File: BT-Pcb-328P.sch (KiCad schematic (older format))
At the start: 18 parts, among them J1 USB_B_Micro, P1 MYSX_2.6, Q1 FDN338P, SW1 1437566-3, U1 AMS1117-3.3, U2 AS312, U3 ATmega328P-AU, U4 RFM69HW

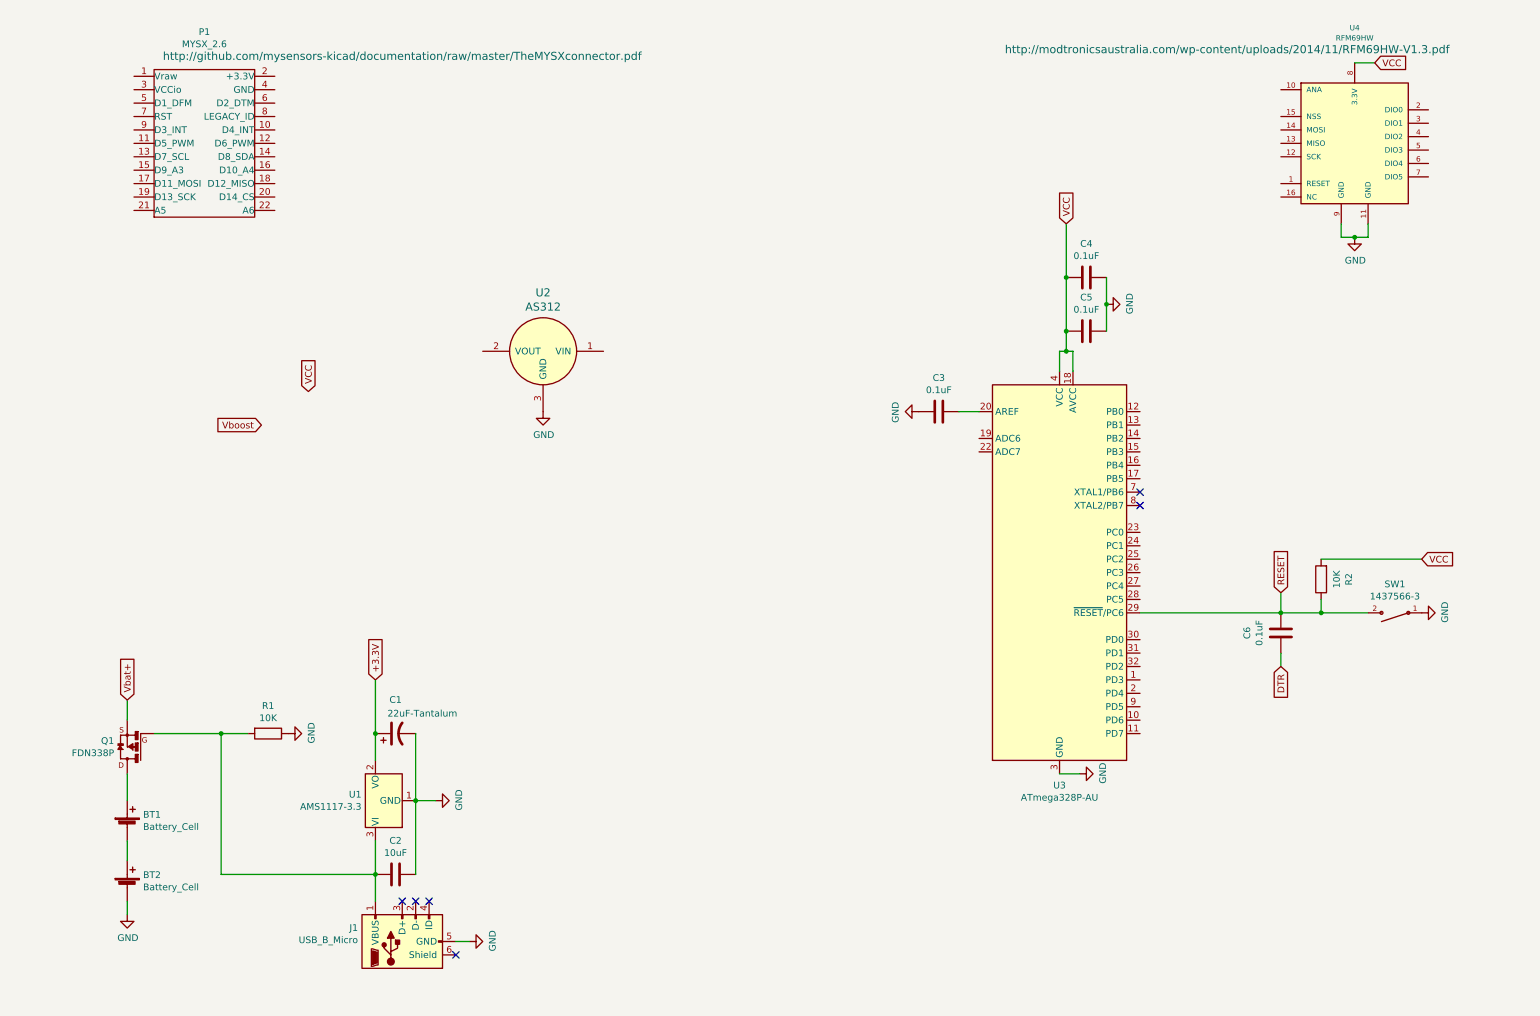
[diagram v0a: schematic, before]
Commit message: Development 2
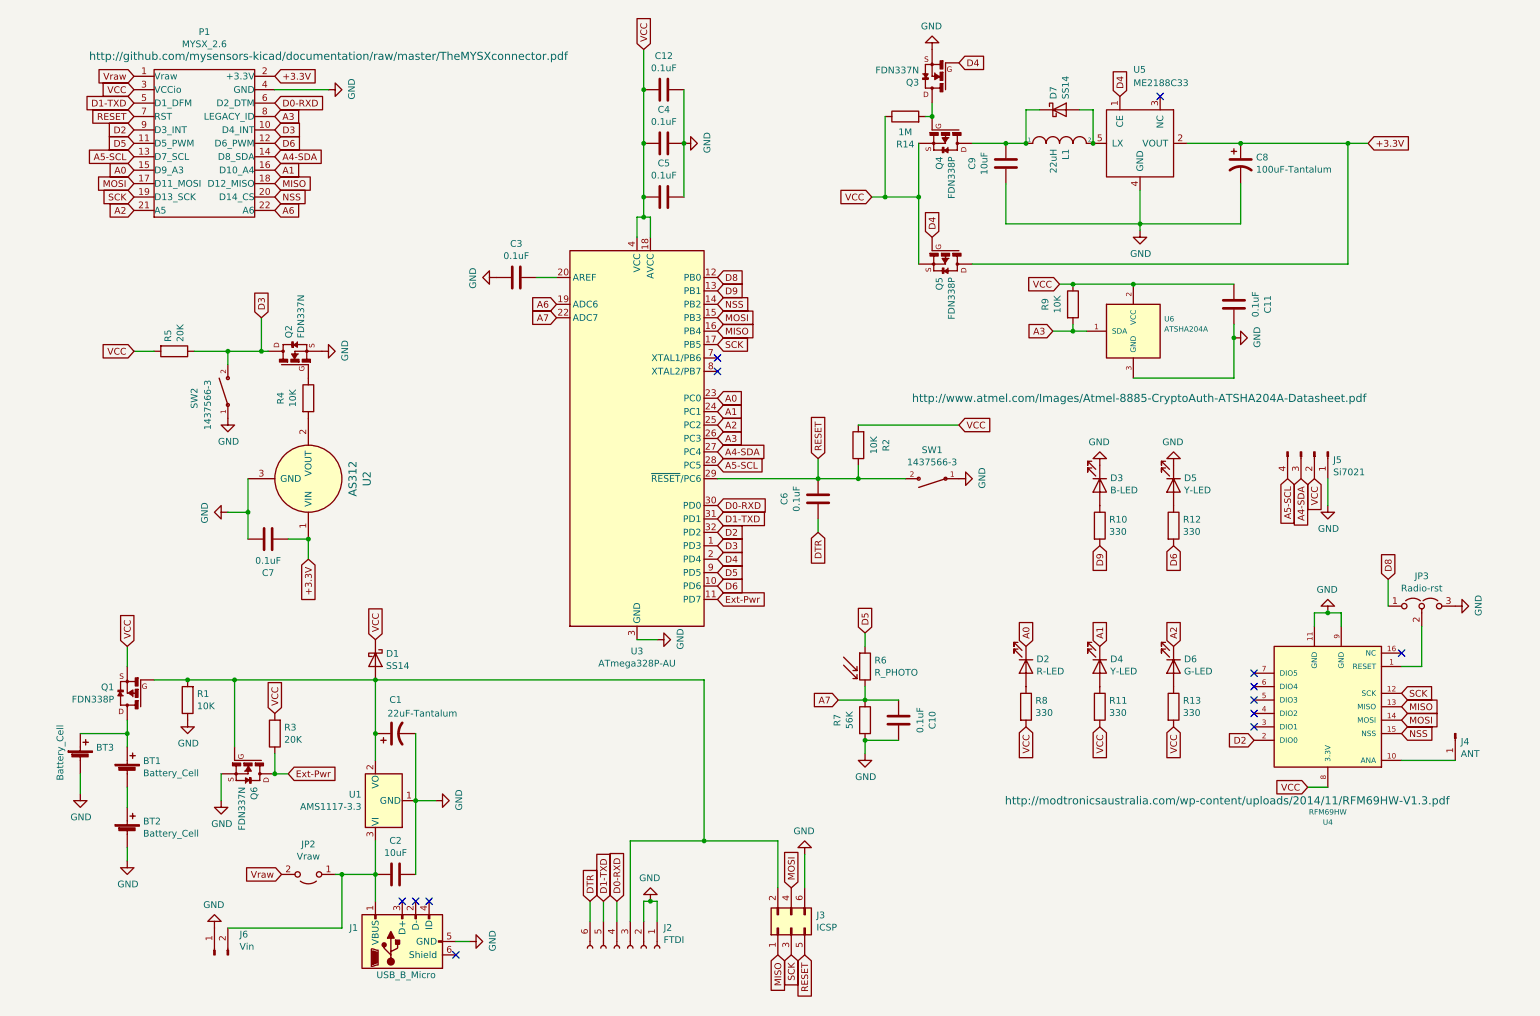
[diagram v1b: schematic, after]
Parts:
- added BT3: Battery_Cell, Battery:BatteryHolder_Keystone_1058_1x2032, symbol Device:Battery_Cell
- added C10, C11, C12, C7: 0.1uF, Capacitor_SMD:C_0805_2012Metric, symbol Device:C
- added C8: 100uF-Tantalum, capacitors:TAJD107K016RNJV, symbol Device:CP1
- added C9: 10uF, Capacitor_SMD:C_0805_2012Metric, symbol Device:C
- added D1, D7: SS14, diodes:SS14, symbol Device:D_Schottky
- added D2: R-LED, LED_SMD:LED_0805_2012Metric, symbol Device:LED
- added D3: B-LED, LED_SMD:LED_0805_2012Metric, symbol Device:LED
- added D4, D5: Y-LED, LED_SMD:LED_0805_2012Metric, symbol Device:LED
- added D6: G-LED, LED_SMD:LED_0805_2012Metric, symbol Device:LED
- added J2: FTDI, Connector_PinSocket_2.54mm:PinSocket_1x06_P2.54mm_Vertical, symbol Connector:Conn_01x06_Female
- added J3: ICSP, Connector_PinHeader_2.54mm:PinHeader_2x03_P2.54mm_Vertical, symbol Connector_Generic:Conn_02x03_Odd_Even
- added J4: ANT, Connector_PinHeader_2.54mm:PinHeader_1x01_P2.54mm_Vertical, symbol Connector:Conn_01x01_Male
- added J5: Si7021, Connector_PinHeader_2.54mm:PinHeader_1x04_P2.54mm_Vertical, symbol Connector:Conn_01x04_Male
- added J6: Vin, Connector_PinHeader_2.54mm:PinHeader_1x02_P2.54mm_Vertical, symbol Connector:Conn_01x02_Male
- added JP2: Vraw, Jumper:SolderJumper-2_P1.3mm_Open_RoundedPad1.0x1.5mm, symbol Jumper:Jumper_2_Open
- added JP3: Radio-rst, Jumper:SolderJumper-3_P1.3mm_Open_RoundedPad1.0x1.5mm_NumberLabels, symbol Jumper:Jumper_3_Open
- added L1: 22uH, Inductor_SMD:L_6.3x6.3_H3, symbol pspice:INDUCTOR
- added Q2, Q3, Q6: FDN337N, FDN337N:SSOT-3, symbol FDN337N:FDN337N
- added Q4, Q5: FDN338P, FDN338P:SSOT-3, symbol FDN338P:FDN338P
- added R10, R11, R12, R13, R8: 330, Resistor_SMD:R_0805_2012Metric, symbol Device:R
- added R14: 1M, Resistor_SMD:R_0805_2012Metric, symbol Device:R
- added R3, R5: 20K, Resistor_SMD:R_0805_2012Metric, symbol Device:R
- added R4, R9: 10K, Resistor_SMD:R_0805_2012Metric, symbol Device:R
- added R6: R_PHOTO, OptoDevice:R_LDR_5.0x4.1mm_P3mm_Vertical, symbol Device:R_PHOTO
- added R7: 56K, Resistor_SMD:R_0805_2012Metric, symbol Device:R
- added SW2: 1437566-3, 1437566-3:SW_1437566-3, symbol 1437566-3:1437566-3
- added U5: ME2188C33, Package_TO_SOT_SMD:SOT-23-5, symbol boost-converters:ME2188C33
- added U6: ATSHA204A, Package_TO_SOT_SMD:SOT-23_Handsoldering, symbol mysensors_security:ATSHA204A
- BT1, BT2: footprint (none) -> batteries:AAA-Keystone-5204-5226-NO-SILK
- C2, C3, C4, C5, C6: footprint (none) -> Capacitor_SMD:C_0805_2012Metric
- J1: footprint (none) -> Connector_USB:USB_Micro-B_Molex-105017-0001
- P1: footprint (none) -> mysensors_connectors:MYSX_2.6
- R1, R2: footprint (none) -> Resistor_SMD:R_0805_2012Metric
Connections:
- net Vbat+ is gone; now on net VCC: Q1.2 (S)
- net +3.3V: now also P1.2 (+3.3V), U2.1 (VIN), C7.2, C8.1, Q5.3 (D), U5.2 (VOUT); no longer C1.1, U1.2 (VO)
- net DTR: now also J2.6 (Pin_6)
- net GND: now also P1.4 (GND), BT3.2 (-), C10.1, C11.1, C12.1, C7.1, C8.2, C9.1, D3.1 (K), D5.1 (K), J2.1 (Pin_1), J2.2 (Pin_2), J3.6 (Pin_6), J5.1 (Pin_1), J6.1 (Pin_1), JP3.3 (B), Q2.2 (S), Q3.2 (S), Q6.2 (S), R7.2, SW2.1, U5.4 (GND), U6.3 (GND)
- net RESET: now also P1.7 (RST), J3.5 (Pin_5)
- net VCC: now also P1.3 (VCCio), C11.2, C12.2, D1.1 (K), J5.2 (Pin_2), Q4.2 (S), Q5.2 (S), R11.2, R13.2, R14.1, R3.2, R5.2, R8.2, R9.1, U6.2 (VCC)
- net at BT1.1 (+), Q1.3 (D): now also BT3.1 (+)
- net at U2.2 (VOUT): now also R4.2
- net at U4.1 (RESET): now also JP3.2 (C)
- net at U4.10 (ANA): now also J4.1 (Pin_1)
- net SCK: now reaches U4.12 (SCK)
- net SCK: now also P1.19 (D13_SCK), U3.17 (PB5), J3.3 (Pin_3)
- net MISO: now reaches U4.13 (MISO)
- net MISO: now also P1.18 (D12_MISO), U3.16 (PB4), J3.1 (Pin_1)
- net MOSI: now reaches U4.14 (MOSI)
- net MOSI: now also P1.17 (D11_MOSI), U3.15 (PB3), J3.4 (Pin_4)
- net NSS: now reaches U4.15 (NSS)
- net NSS: now also P1.20 (D14_CS), U3.14 (PB2)
- net D2: now reaches U4.2 (DIO0)
- net D2: now also P1.9 (D3_INT), U3.32 (PD2)
- net Vraw: now reaches P1.1 (Vraw)
- net Vraw: now also JP2.2 (B)
- net D3: now reaches P1.10 (D4_INT)
- net D3: now also U3.1 (PD3), Q2.3 (D), R5.1, SW2.2
- net D5: now reaches P1.11 (D5_PWM)
- net D5: now also U3.9 (PD5), R6.1
- net D6: now reaches P1.12 (D6_PWM)
- net D6: now also U3.10 (PD6), R12.2
- net A5-SCL: now reaches P1.13 (D7_SCL)
- net A5-SCL: now also U3.28 (PC5), J5.4 (Pin_4)
- net A4-SDA: now reaches P1.14 (D8_SDA)
- net A4-SDA: now also U3.27 (PC4), J5.3 (Pin_3)
- net A0: now reaches P1.15 (D9_A3)
- net A0: now also U3.23 (PC0), D2.1 (K)
- net A1: now reaches P1.16 (D10_A4)
- net A1: now also U3.24 (PC1), D4.1 (K)
- net A2: now reaches P1.21 (A5)
- net A2: now also U3.25 (PC2), D6.1 (K)
- net A6: now reaches P1.22 (A6)
- net A6: now also U3.19 (ADC6)
- net D1-TXD: now reaches P1.5 (D1_DFM)
- net D1-TXD: now also U3.31 (PD1), J2.5 (Pin_5)
- net D0-RXD: now reaches P1.6 (D2_DTM)
- net D0-RXD: now also U3.30 (PD0), J2.4 (Pin_4)
- net A3: now reaches P1.8 (LEGACY_ID)
- net A3: now also U3.26 (PC3), R9.2, U6.1 (SDA)
- net at C2.1, J1.1 (VBUS), U1.3 (VI): now also J6.2 (Pin_2), JP2.1 (A); no longer Q1.1 (G), R1.2
- net Ext-Pwr: now reaches U3.11 (PD7)
- net Ext-Pwr: now also Q6.3 (D), R3.1
- net D8: now reaches U3.12 (PB0)
- net D8: now also JP3.1 (A)
- net D9: now reaches U3.13 (PB1)
- net D9: now also R10.2
- net D4: now reaches U3.2 (PD4)
- net D4: now also Q3.1 (G), Q5.1 (G), U5.1 (CE)
- net A7: now reaches U3.22 (ADC7)
- net A7: now also C10.2, R6.2, R7.1
- new net: C1.1, D1.2 (A), J2.3 (Pin_3), J3.2 (Pin_2), Q1.1 (G), Q6.1 (G), R1.2, U1.2 (VO)
- new net: Q2.1 (G), R4.1
- new net: C9.2, D7.1 (K), L1.1, Q4.3 (D)
- new net: D7.2 (A), L1.2, U5.5 (LX)
- new net: Q3.3 (D), Q4.1 (G), R14.2
- new net: D2.2 (A), R8.1
- new net: D4.2 (A), R11.1
- new net: D6.2 (A), R13.1
- new net: D3.2 (A), R10.1
- new net: D5.2 (A), R12.1
- no-connect marks 6 -> 13
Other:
- moved on the sheet: BT1, BT2, C3, C4, C5, C6, Q1, R2, SW1, U2, U3, U4

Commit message: Development 3
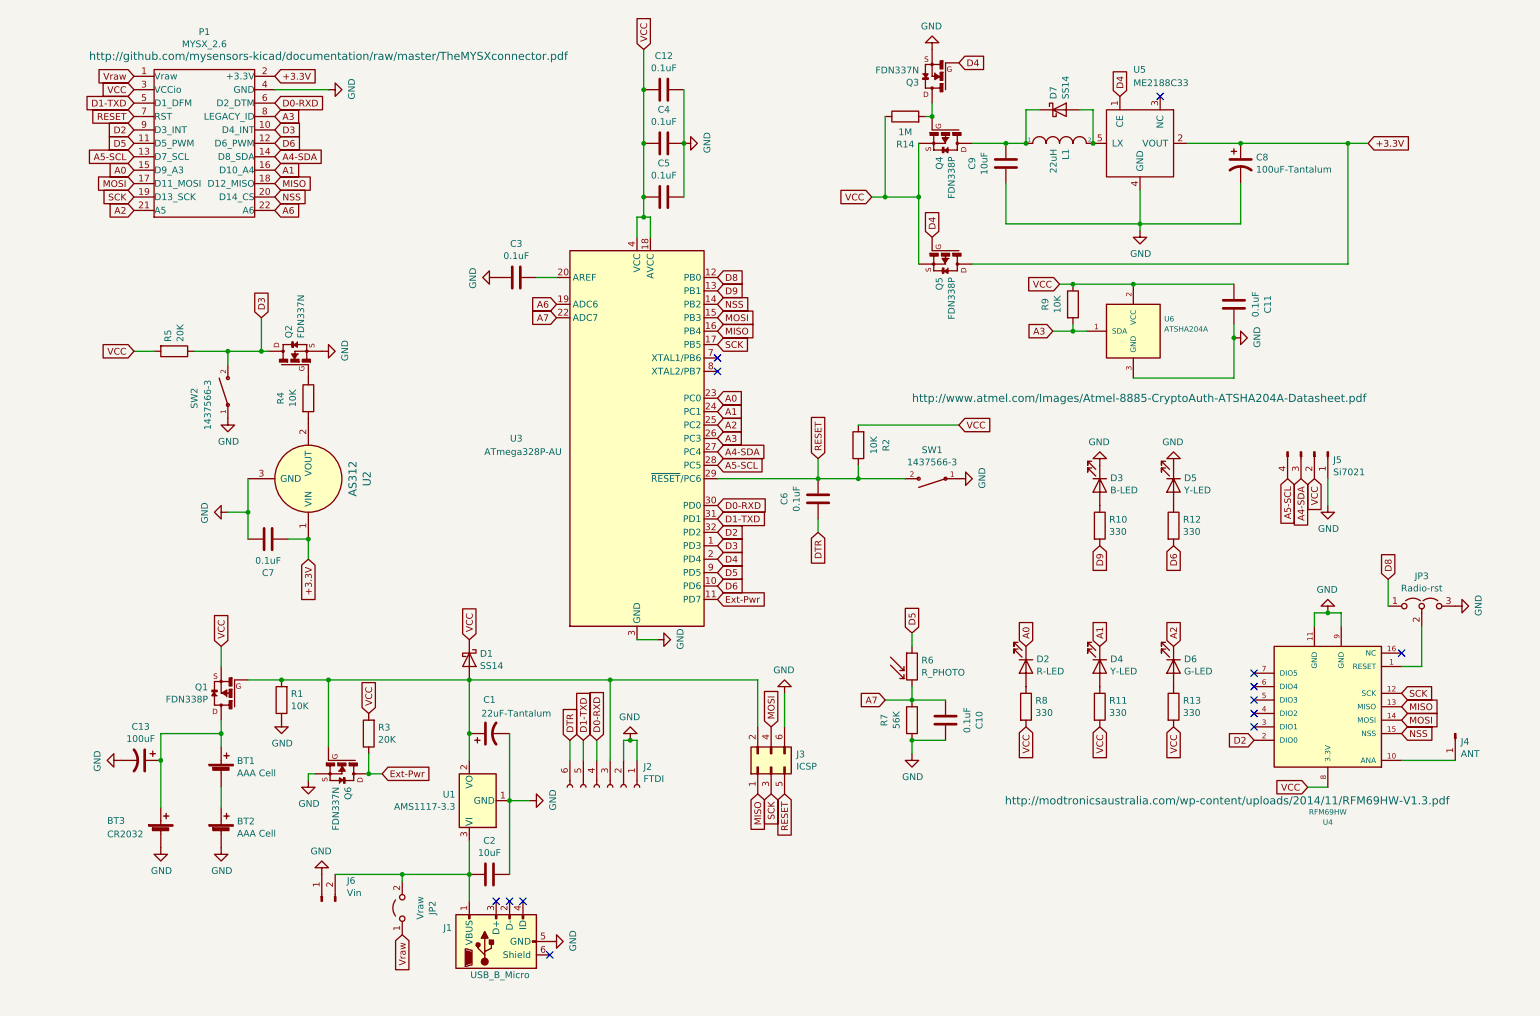
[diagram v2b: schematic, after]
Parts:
- added C13: 100uF, Capacitor_SMD:CP_Elec_6.3x5.4, symbol Device:CP1
- BT1, BT2: value Battery_Cell -> AAA Cell
- BT3: value Battery_Cell -> CR2032
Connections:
- net GND: now also C13.2
- net Vraw: now also JP2.1 (A); no longer JP2.2 (B)
- net at BT1.1 (+), BT3.1 (+), Q1.3 (D): now also C13.1
- net at C2.1, J1.1 (VBUS), J6.2 (Pin_2)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: now also JP2.2 (B); no longer JP2.1 (A)
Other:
- moved on the sheet: BT1, BT2, BT3, C1, C10, C2, D1, J1, J2, J3, J6, JP2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
